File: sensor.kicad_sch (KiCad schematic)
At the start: 278 parts, among them U1 Hall_Sensor, U10 Hall_Sensor, U11 Hall_Sensor, U12 Hall_Sensor, U13 Hall_Sensor, U14 Hall_Sensor, U15 Hall_Sensor, U16 Hall_Sensor, U17 Hall_Sensor, U18 Hall_Sensor, U19 Hall_Sensor, U2 Hall_Sensor, U20 Hall_Sensor, U21 Hall_Sensor, U22 Hall_Sensor, U23 Hall_Sensor, U24 Hall_Sensor, U25 Hall_Sensor, U26 Hall_Sensor, U27 Hall_Sensor, U28 Hall_Sensor, U29 Hall_Sensor, U3 Hall_Sensor, U30 Hall_Sensor, U31 Hall_Sensor, U32 Hall_Sensor, U33 Hall_Sensor, U34 Hall_Sensor, U35 Hall_Sensor, U36 Hall_Sensor, U37 Hall_Sensor, U38 Hall_Sensor, U39 Hall_Sensor, U4 Hall_Sensor, U40 Hall_Sensor, U41 Hall_Sensor, U42 Hall_Sensor, U43 Hall_Sensor, U44 Hall_Sensor, U45 Hall_Sensor, U46 Hall_Sensor, U47 Hall_Sensor, U48 Hall_Sensor, U49 Hall_Sensor, U5 Hall_Sensor, U50 Hall_Sensor, U51 Hall_Sensor, U52 Hall_Sensor, U53 Hall_Sensor, U54 Hall_Sensor, U55 Hall_Sensor, U56 Hall_Sensor, U57 Hall_Sensor, U58 Hall_Sensor, U59 Hall_Sensor, U6 Hall_Sensor, U60 Hall_Sensor, U61 Hall_Sensor, U62 Hall_Sensor, U63 Hall_Sensor, U64 Hall_Sensor, U65 Hall_Sensor, U66 Hall_Sensor, U7 Hall_Sensor, U8 Hall_Sensor, U9 Hall_Sensor

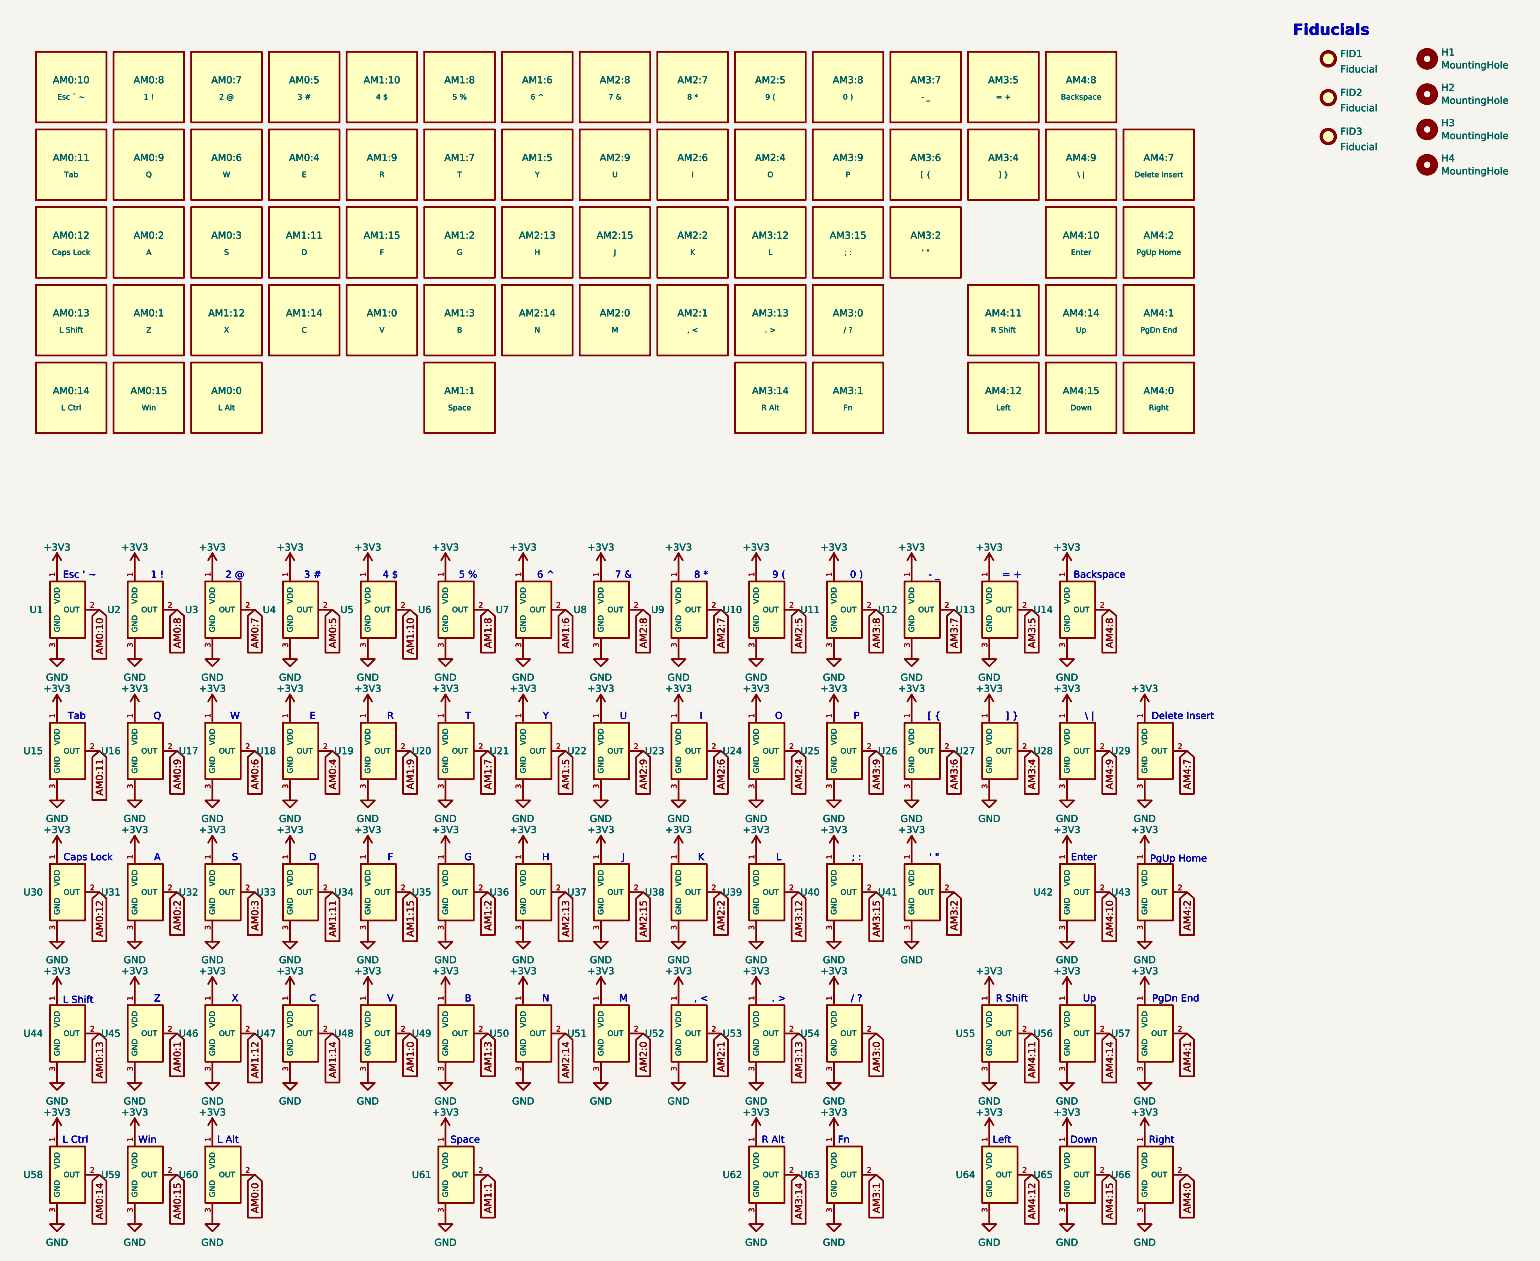
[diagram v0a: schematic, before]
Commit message: Second Commit
new wiring and label
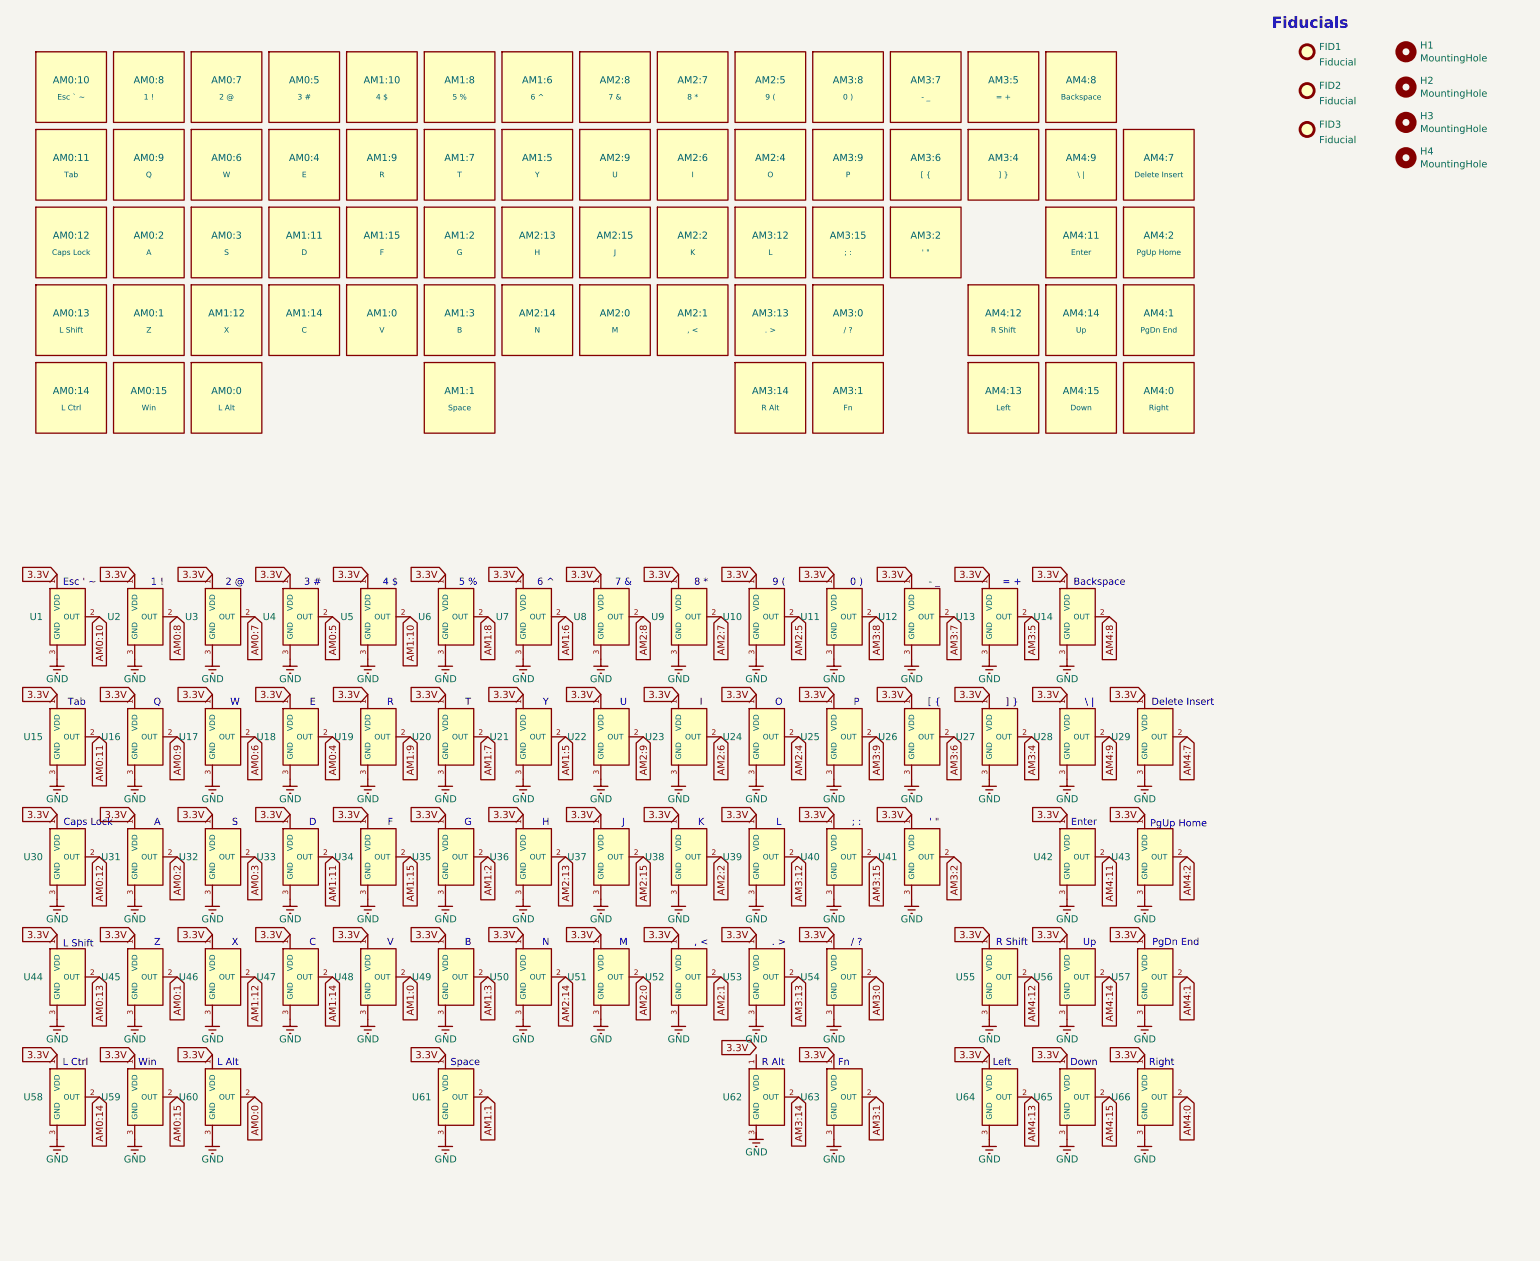
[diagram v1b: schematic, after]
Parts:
- removed AM0:0 (x2): L Alt, HE_Keyswitch:MX_Gateron_HE_1.25u, symbol voidswitch:VoidSwitch
- removed AM0:1 (x2): Z, HE_Keyswitch:MX_Gateron_HE_1u, symbol voidswitch:VoidSwitch
- removed AM0:10 (x2): Esc ` ~, HE_Keyswitch:MX_Gateron_HE_1u, symbol voidswitch:VoidSwitch
- removed AM0:11 (x2): Tab, HE_Keyswitch:MX_Gateron_HE_1.5u, symbol voidswitch:VoidSwitch
- removed AM0:12 (x2): Caps Lock, HE_Keyswitch:MX_Gateron_HE_1.75u, symbol voidswitch:VoidSwitch
- removed AM0:13 (x2): L Shift, HE_Keyswitch:MX_Gateron_HE_2.25u_Stab, symbol voidswitch:VoidSwitch
- removed AM0:14 (x2): L Ctrl, HE_Keyswitch:MX_Gateron_HE_1.25u, symbol voidswitch:VoidSwitch
- removed AM0:15 (x2): Win, HE_Keyswitch:MX_Gateron_HE_1.25u, symbol voidswitch:VoidSwitch
- removed AM0:2 (x2): A, HE_Keyswitch:MX_Gateron_HE_1u, symbol voidswitch:VoidSwitch
- removed AM0:3 (x2): S, HE_Keyswitch:MX_Gateron_HE_1u, symbol voidswitch:VoidSwitch
- removed AM0:4 (x2): E, HE_Keyswitch:MX_Gateron_HE_1u, symbol voidswitch:VoidSwitch
- removed AM0:5 (x2): 3 #, HE_Keyswitch:MX_Gateron_HE_1u, symbol voidswitch:VoidSwitch
- removed AM0:6 (x2): W, HE_Keyswitch:MX_Gateron_HE_1u, symbol voidswitch:VoidSwitch
- removed AM0:7 (x2): 2 @, HE_Keyswitch:MX_Gateron_HE_1u, symbol voidswitch:VoidSwitch
- removed AM0:8 (x2): 1 !, HE_Keyswitch:MX_Gateron_HE_1u, symbol voidswitch:VoidSwitch
- removed AM0:9 (x2): Q, HE_Keyswitch:MX_Gateron_HE_1u, symbol voidswitch:VoidSwitch
- removed AM1:0 (x2): V, HE_Keyswitch:MX_Gateron_HE_1u, symbol voidswitch:VoidSwitch
- removed AM1:1 (x2): Space, HE_Keyswitch:MX_Gateron_HE_6.25u_Stab, symbol voidswitch:VoidSwitch
- removed AM1:10 (x2): 4 $, HE_Keyswitch:MX_Gateron_HE_1u, symbol voidswitch:VoidSwitch
- removed AM1:11 (x2): D, HE_Keyswitch:MX_Gateron_HE_1u, symbol voidswitch:VoidSwitch
- removed AM1:12 (x2): X, HE_Keyswitch:MX_Gateron_HE_1u, symbol voidswitch:VoidSwitch
- removed AM1:14 (x2): C, HE_Keyswitch:MX_Gateron_HE_1u, symbol voidswitch:VoidSwitch
- removed AM1:15 (x2): F, HE_Keyswitch:MX_Gateron_HE_1u, symbol voidswitch:VoidSwitch
- removed AM1:2 (x2): G, HE_Keyswitch:MX_Gateron_HE_1u, symbol voidswitch:VoidSwitch
- removed AM1:3 (x2): B, HE_Keyswitch:MX_Gateron_HE_1u, symbol voidswitch:VoidSwitch
- removed AM1:5 (x2): Y, HE_Keyswitch:MX_Gateron_HE_1u, symbol voidswitch:VoidSwitch
- removed AM1:6 (x2): 6 ^, HE_Keyswitch:MX_Gateron_HE_1u, symbol voidswitch:VoidSwitch
- removed AM1:7 (x2): T, HE_Keyswitch:MX_Gateron_HE_1u, symbol voidswitch:VoidSwitch
- removed AM1:8 (x2): 5 %, HE_Keyswitch:MX_Gateron_HE_1u, symbol voidswitch:VoidSwitch
- removed AM1:9 (x2): R, HE_Keyswitch:MX_Gateron_HE_1u, symbol voidswitch:VoidSwitch
- removed AM2:0 (x2): M, HE_Keyswitch:MX_Gateron_HE_1u, symbol voidswitch:VoidSwitch
- removed AM2:1 (x2): , <, HE_Keyswitch:MX_Gateron_HE_1u, symbol voidswitch:VoidSwitch
- removed AM2:13 (x2): H, HE_Keyswitch:MX_Gateron_HE_1u, symbol voidswitch:VoidSwitch
- removed AM2:14 (x2): N, HE_Keyswitch:MX_Gateron_HE_1u, symbol voidswitch:VoidSwitch
- removed AM2:15 (x2): J, HE_Keyswitch:MX_Gateron_HE_1u, symbol voidswitch:VoidSwitch
- removed AM2:2 (x2): K, HE_Keyswitch:MX_Gateron_HE_1u, symbol voidswitch:VoidSwitch
- removed AM2:4 (x2): O, HE_Keyswitch:MX_Gateron_HE_1u, symbol voidswitch:VoidSwitch
- removed AM2:5 (x2): 9 (, HE_Keyswitch:MX_Gateron_HE_1u, symbol voidswitch:VoidSwitch
- removed AM2:6 (x2): I, HE_Keyswitch:MX_Gateron_HE_1u, symbol voidswitch:VoidSwitch
- removed AM2:7 (x2): 8 *, HE_Keyswitch:MX_Gateron_HE_1u, symbol voidswitch:VoidSwitch
- removed AM2:8 (x2): 7 &, HE_Keyswitch:MX_Gateron_HE_1u, symbol voidswitch:VoidSwitch
- removed AM2:9 (x2): U, HE_Keyswitch:MX_Gateron_HE_1u, symbol voidswitch:VoidSwitch
- removed AM3:0 (x2): / ?, HE_Keyswitch:MX_Gateron_HE_1u, symbol voidswitch:VoidSwitch
- removed AM3:1 (x2): Fn, HE_Keyswitch:MX_Gateron_HE_1.25u, symbol voidswitch:VoidSwitch
- removed AM3:12 (x2): L, HE_Keyswitch:MX_Gateron_HE_1u, symbol voidswitch:VoidSwitch
- removed AM3:13 (x2): . >, HE_Keyswitch:MX_Gateron_HE_1u, symbol voidswitch:VoidSwitch
- removed AM3:14 (x2): R Alt, HE_Keyswitch:MX_Gateron_HE_1.25u, symbol voidswitch:VoidSwitch
- removed AM3:15 (x2): ; :, HE_Keyswitch:MX_Gateron_HE_1u, symbol voidswitch:VoidSwitch
- removed AM3:2 (x2): ' ", HE_Keyswitch:MX_Gateron_HE_1u, symbol voidswitch:VoidSwitch
- removed AM3:4 (x2): ] }, HE_Keyswitch:MX_Gateron_HE_1u, symbol voidswitch:VoidSwitch
- removed AM3:5 (x2): = +, HE_Keyswitch:MX_Gateron_HE_1u, symbol voidswitch:VoidSwitch
- removed AM3:6 (x2): [ {, HE_Keyswitch:MX_Gateron_HE_1u, symbol voidswitch:VoidSwitch
- removed AM3:7 (x2): - _, HE_Keyswitch:MX_Gateron_HE_1u, symbol voidswitch:VoidSwitch
- removed AM3:8 (x2): 0 ), HE_Keyswitch:MX_Gateron_HE_1u, symbol voidswitch:VoidSwitch
- removed AM3:9 (x2): P, HE_Keyswitch:MX_Gateron_HE_1u, symbol voidswitch:VoidSwitch
- removed AM4:0 (x2): Right, HE_Keyswitch:MX_Gateron_HE_1u, symbol voidswitch:VoidSwitch
- removed AM4:1 (x2): PgDn End, HE_Keyswitch:MX_Gateron_HE_1u, symbol voidswitch:VoidSwitch
- removed AM4:10 (x2): Enter, HE_Keyswitch:MX_Gateron_HE_2.25u_Stab, symbol voidswitch:VoidSwitch
- removed AM4:11 (x2): R Shift, HE_Keyswitch:MX_Gateron_HE_1.75u, symbol voidswitch:VoidSwitch
- removed AM4:12 (x2): Left, HE_Keyswitch:MX_Gateron_HE_1u, symbol voidswitch:VoidSwitch
- removed AM4:14 (x2): Up, HE_Keyswitch:MX_Gateron_HE_1u, symbol voidswitch:VoidSwitch
- removed AM4:15 (x2): Down, HE_Keyswitch:MX_Gateron_HE_1u, symbol voidswitch:VoidSwitch
- removed AM4:2 (x2): PgUp Home, HE_Keyswitch:MX_Gateron_HE_1u, symbol voidswitch:VoidSwitch
- removed AM4:7 (x2): Delete Insert, HE_Keyswitch:MX_Gateron_HE_1u, symbol voidswitch:VoidSwitch
- removed AM4:8 (x2): Backspace, HE_Keyswitch:MX_Gateron_HE_2u_Stab, symbol voidswitch:VoidSwitch
- removed AM4:9 (x2): \ |, HE_Keyswitch:MX_Gateron_HE_1.5u, symbol voidswitch:VoidSwitch
- removed FID1 (x2), FID2 (x2), FID3 (x2): Fiducial, Fiducial:Fiducial_1mm_Mask2mm, symbol Mechanical:Fiducial
- removed H1 (x2), H2 (x2), H3 (x2), H4 (x2): MountingHole, MountingHole:MountingHole_3.2mm_M3_Pad, symbol Mechanical:MountingHole
- removed U1 (x2), U10 (x2), U11 (x2), U12 (x2), U13 (x2), U14 (x2), U15 (x2), U16 (x2), U17 (x2), U18 (x2), U19 (x2), U2 (x2), U20 (x2), U21 (x2), U22 (x2), U23 (x2), U24 (x2), U25 (x2), U26 (x2), U27 (x2), U28 (x2), U29 (x2), U3 (x2), U30 (x2), U31 (x2), U32 (x2), U33 (x2), U34 (x2), U35 (x2), U36 (x2), U37 (x2), U38 (x2), U39 (x2), U4 (x2), U40 (x2), U41 (x2), U42 (x2), U43 (x2), U44 (x2), U45 (x2), U46 (x2), U47 (x2), U48 (x2), U49 (x2), U5 (x2), U50 (x2), U51 (x2), U52 (x2), U53 (x2), U54 (x2), U55 (x2), U56 (x2), U57 (x2), U58 (x2), U59 (x2), U6 (x2), U60 (x2), U61 (x2), U62 (x2), U63 (x2), U64 (x2), U65 (x2), U66 (x2), U7 (x2), U8 (x2), U9 (x2): Hall_Sensor, Package_TO_SOT_SMD:SOT-23, symbol 49e:Hall_Sensor
- added AM0:0: L Alt, HE_Keyswitch:MX_Gateron_HE_1.25u, symbol voidswitch:VoidSwitch
- added AM0:1: Z, HE_Keyswitch:MX_Gateron_HE_1u, symbol voidswitch:VoidSwitch
- added AM0:10: Esc ` ~, HE_Keyswitch:MX_Gateron_HE_1u, symbol voidswitch:VoidSwitch
- added AM0:11: Tab, HE_Keyswitch:MX_Gateron_HE_1.5u, symbol voidswitch:VoidSwitch
- added AM0:12: Caps Lock, HE_Keyswitch:MX_Gateron_HE_1.75u, symbol voidswitch:VoidSwitch
- added AM0:13: L Shift, HE_Keyswitch:MX_Gateron_HE_2.25u_Stab, symbol voidswitch:VoidSwitch
- added AM0:14: L Ctrl, HE_Keyswitch:MX_Gateron_HE_1.25u, symbol voidswitch:VoidSwitch
- added AM0:15: Win, HE_Keyswitch:MX_Gateron_HE_1.25u, symbol voidswitch:VoidSwitch
- added AM0:2: A, HE_Keyswitch:MX_Gateron_HE_1u, symbol voidswitch:VoidSwitch
- added AM0:3: S, HE_Keyswitch:MX_Gateron_HE_1u, symbol voidswitch:VoidSwitch
- added AM0:4: E, HE_Keyswitch:MX_Gateron_HE_1u, symbol voidswitch:VoidSwitch
- added AM0:5: 3 #, HE_Keyswitch:MX_Gateron_HE_1u, symbol voidswitch:VoidSwitch
- added AM0:6: W, HE_Keyswitch:MX_Gateron_HE_1u, symbol voidswitch:VoidSwitch
- added AM0:7: 2 @, HE_Keyswitch:MX_Gateron_HE_1u, symbol voidswitch:VoidSwitch
- added AM0:8: 1 !, HE_Keyswitch:MX_Gateron_HE_1u, symbol voidswitch:VoidSwitch
- added AM0:9: Q, HE_Keyswitch:MX_Gateron_HE_1u, symbol voidswitch:VoidSwitch
- added AM1:0: V, HE_Keyswitch:MX_Gateron_HE_1u, symbol voidswitch:VoidSwitch
- added AM1:1: Space, HE_Keyswitch:MX_Gateron_HE_6.25u_Stab, symbol voidswitch:VoidSwitch
- added AM1:10: 4 $, HE_Keyswitch:MX_Gateron_HE_1u, symbol voidswitch:VoidSwitch
- added AM1:11: D, HE_Keyswitch:MX_Gateron_HE_1u, symbol voidswitch:VoidSwitch
- added AM1:12: X, HE_Keyswitch:MX_Gateron_HE_1u, symbol voidswitch:VoidSwitch
- added AM1:14: C, HE_Keyswitch:MX_Gateron_HE_1u, symbol voidswitch:VoidSwitch
- added AM1:15: F, HE_Keyswitch:MX_Gateron_HE_1u, symbol voidswitch:VoidSwitch
- added AM1:2: G, HE_Keyswitch:MX_Gateron_HE_1u, symbol voidswitch:VoidSwitch
- added AM1:3: B, HE_Keyswitch:MX_Gateron_HE_1u, symbol voidswitch:VoidSwitch
- added AM1:5: Y, HE_Keyswitch:MX_Gateron_HE_1u, symbol voidswitch:VoidSwitch
- added AM1:6: 6 ^, HE_Keyswitch:MX_Gateron_HE_1u, symbol voidswitch:VoidSwitch
- added AM1:7: T, HE_Keyswitch:MX_Gateron_HE_1u, symbol voidswitch:VoidSwitch
- added AM1:8: 5 %, HE_Keyswitch:MX_Gateron_HE_1u, symbol voidswitch:VoidSwitch
- added AM1:9: R, HE_Keyswitch:MX_Gateron_HE_1u, symbol voidswitch:VoidSwitch
- added AM2:0: M, HE_Keyswitch:MX_Gateron_HE_1u, symbol voidswitch:VoidSwitch
- added AM2:1: , <, HE_Keyswitch:MX_Gateron_HE_1u, symbol voidswitch:VoidSwitch
- added AM2:13: H, HE_Keyswitch:MX_Gateron_HE_1u, symbol voidswitch:VoidSwitch
- added AM2:14: N, HE_Keyswitch:MX_Gateron_HE_1u, symbol voidswitch:VoidSwitch
- added AM2:15: J, HE_Keyswitch:MX_Gateron_HE_1u, symbol voidswitch:VoidSwitch
- added AM2:2: K, HE_Keyswitch:MX_Gateron_HE_1u, symbol voidswitch:VoidSwitch
- added AM2:4: O, HE_Keyswitch:MX_Gateron_HE_1u, symbol voidswitch:VoidSwitch
- added AM2:5: 9 (, HE_Keyswitch:MX_Gateron_HE_1u, symbol voidswitch:VoidSwitch
- added AM2:6: I, HE_Keyswitch:MX_Gateron_HE_1u, symbol voidswitch:VoidSwitch
- added AM2:7: 8 *, HE_Keyswitch:MX_Gateron_HE_1u, symbol voidswitch:VoidSwitch
- added AM2:8: 7 &, HE_Keyswitch:MX_Gateron_HE_1u, symbol voidswitch:VoidSwitch
- added AM2:9: U, HE_Keyswitch:MX_Gateron_HE_1u, symbol voidswitch:VoidSwitch
- added AM3:0: / ?, HE_Keyswitch:MX_Gateron_HE_1u, symbol voidswitch:VoidSwitch
- added AM3:1: Fn, HE_Keyswitch:MX_Gateron_HE_1.25u, symbol voidswitch:VoidSwitch
- added AM3:12: L, HE_Keyswitch:MX_Gateron_HE_1u, symbol voidswitch:VoidSwitch
- added AM3:13: . >, HE_Keyswitch:MX_Gateron_HE_1u, symbol voidswitch:VoidSwitch
- added AM3:14: R Alt, HE_Keyswitch:MX_Gateron_HE_1.25u, symbol voidswitch:VoidSwitch
- added AM3:15: ; :, HE_Keyswitch:MX_Gateron_HE_1u, symbol voidswitch:VoidSwitch
- added AM3:2: ' ", HE_Keyswitch:MX_Gateron_HE_1u, symbol voidswitch:VoidSwitch
- added AM3:4: ] }, HE_Keyswitch:MX_Gateron_HE_1u, symbol voidswitch:VoidSwitch
- added AM3:5: = +, HE_Keyswitch:MX_Gateron_HE_1u, symbol voidswitch:VoidSwitch
- added AM3:6: [ {, HE_Keyswitch:MX_Gateron_HE_1u, symbol voidswitch:VoidSwitch
- added AM3:7: - _, HE_Keyswitch:MX_Gateron_HE_1u, symbol voidswitch:VoidSwitch
- added AM3:8: 0 ), HE_Keyswitch:MX_Gateron_HE_1u, symbol voidswitch:VoidSwitch
- added AM3:9: P, HE_Keyswitch:MX_Gateron_HE_1u, symbol voidswitch:VoidSwitch
- added AM4:0: Right, HE_Keyswitch:MX_Gateron_HE_1u, symbol voidswitch:VoidSwitch
- added AM4:1: PgDn End, HE_Keyswitch:MX_Gateron_HE_1u, symbol voidswitch:VoidSwitch
- added AM4:11: Enter, HE_Keyswitch:MX_Gateron_HE_2.25u_Stab, symbol voidswitch:VoidSwitch
- added AM4:12: R Shift, HE_Keyswitch:MX_Gateron_HE_1.75u, symbol voidswitch:VoidSwitch
- added AM4:13: Left, HE_Keyswitch:MX_Gateron_HE_1u, symbol voidswitch:VoidSwitch
- added AM4:14: Up, HE_Keyswitch:MX_Gateron_HE_1u, symbol voidswitch:VoidSwitch
- added AM4:15: Down, HE_Keyswitch:MX_Gateron_HE_1u, symbol voidswitch:VoidSwitch
- added AM4:2: PgUp Home, HE_Keyswitch:MX_Gateron_HE_1u, symbol voidswitch:VoidSwitch
- added AM4:7: Delete Insert, HE_Keyswitch:MX_Gateron_HE_1u, symbol voidswitch:VoidSwitch
- added AM4:8: Backspace, HE_Keyswitch:MX_Gateron_HE_2u_Stab, symbol voidswitch:VoidSwitch
- added AM4:9: \ |, HE_Keyswitch:MX_Gateron_HE_1.5u, symbol voidswitch:VoidSwitch
- added FID1, FID2, FID3: Fiducial, Fiducial:Fiducial_1mm_Mask2mm, symbol Mechanical:Fiducial
- added H1, H2, H3, H4: MountingHole, MountingHole:MountingHole_3.2mm_M3_Pad, symbol Mechanical:MountingHole
- added U1, U10, U11, U12, U13, U14, U15, U16, U17, U18, U19, U2, U20, U21, U22, U23, U24, U25, U26, U27, U28, U29, U3, U30, U31, U32, U33, U34, U35, U36, U37, U38, U39, U4, U40, U41, U42, U43, U44, U45, U46, U47, U48, U49, U5, U50, U51, U52, U53, U54, U55, U56, U57, U58, U59, U6, U60, U61, U62, U63, U64, U65, U66, U7, U8, U9: Hall_Sensor, Package_TO_SOT_SMD:SOT-23, symbol 49e:Hall_Sensor
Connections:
- net AM0:0: now also U60.2 (OUT)
- net AM0:1: now also U45.2 (OUT)
- net AM0:10: now also U1.2 (OUT)
- net AM0:11: now also U15.2 (OUT)
- net AM0:12: now also U30.2 (OUT)
- net AM0:13: now also U44.2 (OUT)
- net AM0:14: now also U58.2 (OUT)
- net AM0:15: now also U59.2 (OUT)
- net AM0:2: now also U31.2 (OUT)
- net AM0:3: now also U32.2 (OUT)
- net AM0:4: now also U18.2 (OUT)
- net AM0:5: now also U4.2 (OUT)
- net AM0:6: now also U17.2 (OUT)
- net AM0:7: now also U3.2 (OUT)
- net AM0:8: now also U2.2 (OUT)
- net AM0:9: now also U16.2 (OUT)
- net AM1:0: now also U48.2 (OUT)
- net AM1:1: now also U61.2 (OUT)
- net AM1:10: now also U5.2 (OUT)
- net AM1:11: now also U33.2 (OUT)
- net AM1:12: now also U46.2 (OUT)
- net AM1:14: now also U47.2 (OUT)
- net AM1:15: now also U34.2 (OUT)
- net AM1:2: now also U35.2 (OUT)
- net AM1:3: now also U49.2 (OUT)
- net AM1:5: now also U21.2 (OUT)
- net AM1:6: now also U7.2 (OUT)
- net AM1:7: now also U20.2 (OUT)
- net AM1:8: now also U6.2 (OUT)
- net AM1:9: now also U19.2 (OUT)
- net AM2:0: now also U51.2 (OUT)
- net AM2:1: now also U52.2 (OUT)
- net AM2:13: now also U36.2 (OUT)
- net AM2:14: now also U50.2 (OUT)
- net AM2:15: now also U37.2 (OUT)
- net AM2:2: now also U38.2 (OUT)
- net AM2:4: now also U24.2 (OUT)
- net AM2:5: now also U10.2 (OUT)
- net AM2:6: now also U23.2 (OUT)
- net AM2:7: now also U9.2 (OUT)
- net AM2:8: now also U8.2 (OUT)
- net AM2:9: now also U22.2 (OUT)
- net AM3:0: now also U54.2 (OUT)
- net AM3:1: now also U63.2 (OUT)
- net AM3:12: now also U39.2 (OUT)
- net AM3:13: now also U53.2 (OUT)
- net AM3:14: now also U62.2 (OUT)
- net AM3:15: now also U40.2 (OUT)
- net AM3:2: now also U41.2 (OUT)
- net AM3:4: now also U27.2 (OUT)
- net AM3:5: now also U13.2 (OUT)
- net AM3:6: now also U26.2 (OUT)
- net AM3:7: now also U12.2 (OUT)
- net AM3:8: now also U11.2 (OUT)
- net AM3:9: now also U25.2 (OUT)
- net AM4:0: now also U66.2 (OUT)
- net AM4:1: now also U57.2 (OUT)
- net AM4:11: now also U42.2 (OUT)
- net AM4:12: now also U55.2 (OUT)
- net AM4:14: now also U56.2 (OUT)
- net AM4:15: now also U65.2 (OUT)
- net AM4:2: now also U43.2 (OUT)
- net AM4:7: now also U29.2 (OUT)
- net AM4:8: now also U14.2 (OUT)
- net AM4:9: now also U28.2 (OUT)
- net GND: now also U1.3 (GND), U10.3 (GND), U11.3 (GND), U12.3 (GND), U13.3 (GND), U14.3 (GND), U15.3 (GND), U16.3 (GND), U17.3 (GND), U18.3 (GND), U19.3 (GND), U2.3 (GND), U20.3 (GND), U21.3 (GND), U22.3 (GND), U23.3 (GND), U24.3 (GND), U25.3 (GND), U26.3 (GND), U27.3 (GND), U28.3 (GND), U29.3 (GND), U3.3 (GND), U30.3 (GND), U31.3 (GND), U32.3 (GND), U33.3 (GND), U34.3 (GND), U35.3 (GND), U36.3 (GND), U37.3 (GND), U38.3 (GND), U39.3 (GND), U4.3 (GND), U40.3 (GND), U41.3 (GND), U42.3 (GND), U43.3 (GND), U44.3 (GND), U45.3 (GND), U46.3 (GND), U47.3 (GND), U48.3 (GND), U49.3 (GND), U5.3 (GND), U50.3 (GND), U51.3 (GND), U52.3 (GND), U53.3 (GND), U54.3 (GND), U55.3 (GND), U56.3 (GND), U57.3 (GND), U58.3 (GND), U59.3 (GND), U6.3 (GND), U60.3 (GND), U61.3 (GND), U63.3 (GND), U64.3 (GND), U65.3 (GND), U66.3 (GND), U7.3 (GND), U8.3 (GND), U9.3 (GND)
- new net 3.3V: U1.1 (VDD), U10.1 (VDD), U11.1 (VDD), U12.1 (VDD), U13.1 (VDD), U14.1 (VDD), U15.1 (VDD), U16.1 (VDD), U17.1 (VDD), U18.1 (VDD), U19.1 (VDD), U2.1 (VDD), U20.1 (VDD), U21.1 (VDD), U22.1 (VDD), U23.1 (VDD), U24.1 (VDD), U25.1 (VDD), U26.1 (VDD), U27.1 (VDD), U28.1 (VDD), U29.1 (VDD), U3.1 (VDD), U30.1 (VDD), U31.1 (VDD), U32.1 (VDD), U33.1 (VDD), U34.1 (VDD), U35.1 (VDD), U36.1 (VDD), U37.1 (VDD), U38.1 (VDD), U39.1 (VDD), U4.1 (VDD), U40.1 (VDD), U41.1 (VDD), U42.1 (VDD), U43.1 (VDD), U44.1 (VDD), U45.1 (VDD), U46.1 (VDD), U47.1 (VDD), U48.1 (VDD), U49.1 (VDD), U5.1 (VDD), U50.1 (VDD), U51.1 (VDD), U52.1 (VDD), U53.1 (VDD), U54.1 (VDD), U55.1 (VDD), U56.1 (VDD), U57.1 (VDD), U58.1 (VDD), U59.1 (VDD), U6.1 (VDD), U60.1 (VDD), U61.1 (VDD), U63.1 (VDD), U64.1 (VDD), U65.1 (VDD), U66.1 (VDD), U7.1 (VDD), U8.1 (VDD), U9.1 (VDD)
- new net AM4:13: U64.2 (OUT)
